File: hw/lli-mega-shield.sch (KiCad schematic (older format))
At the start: 39 parts

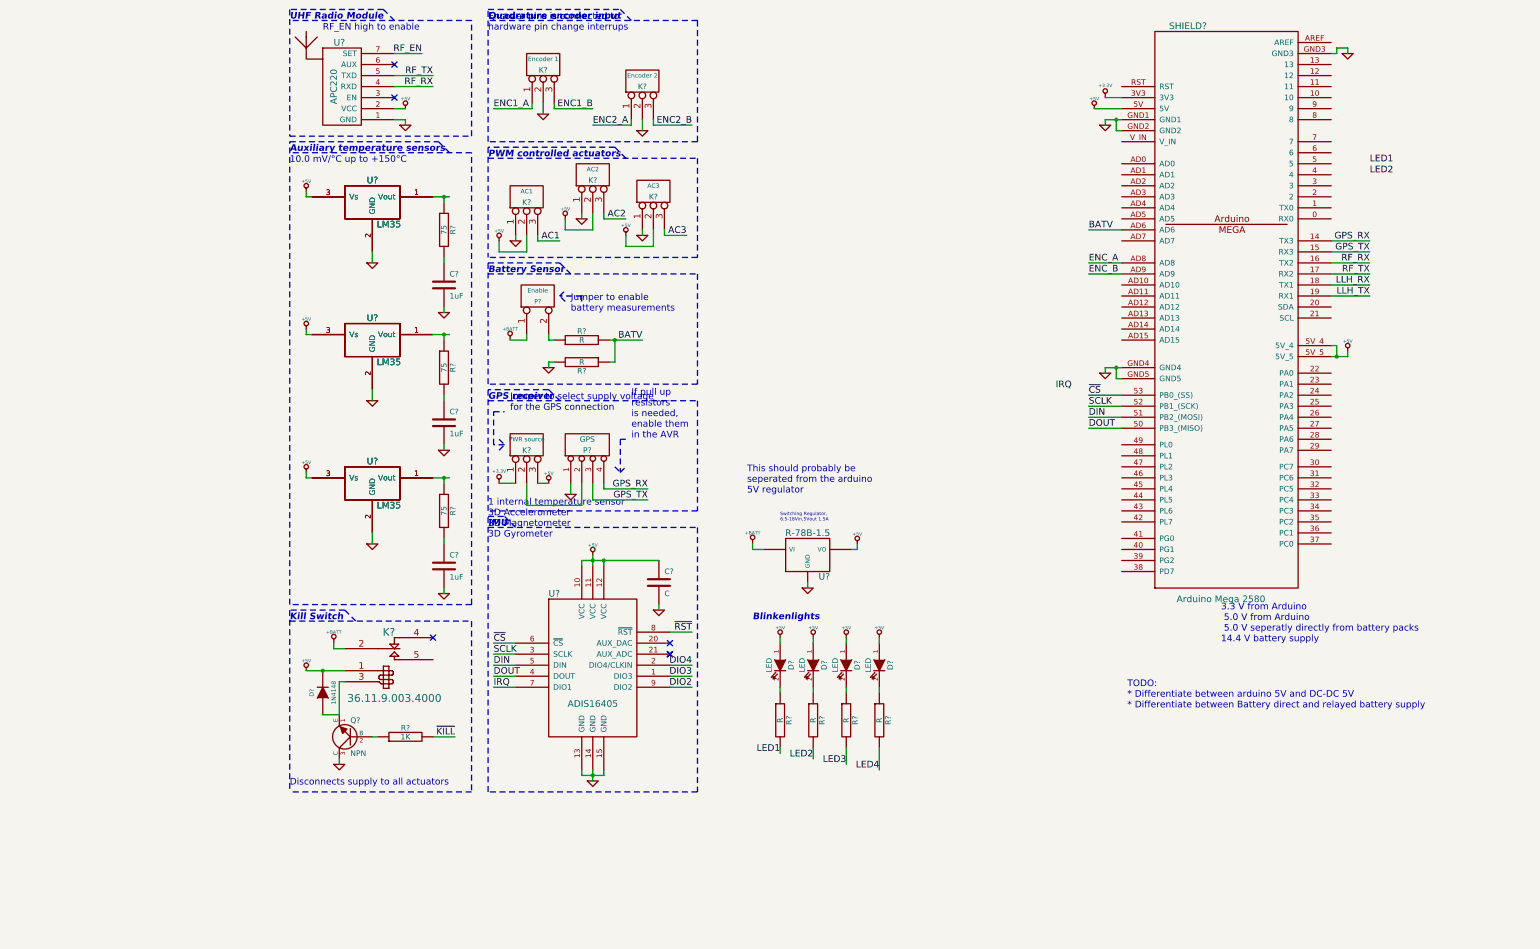
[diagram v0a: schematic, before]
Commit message: That must be hardware enough today
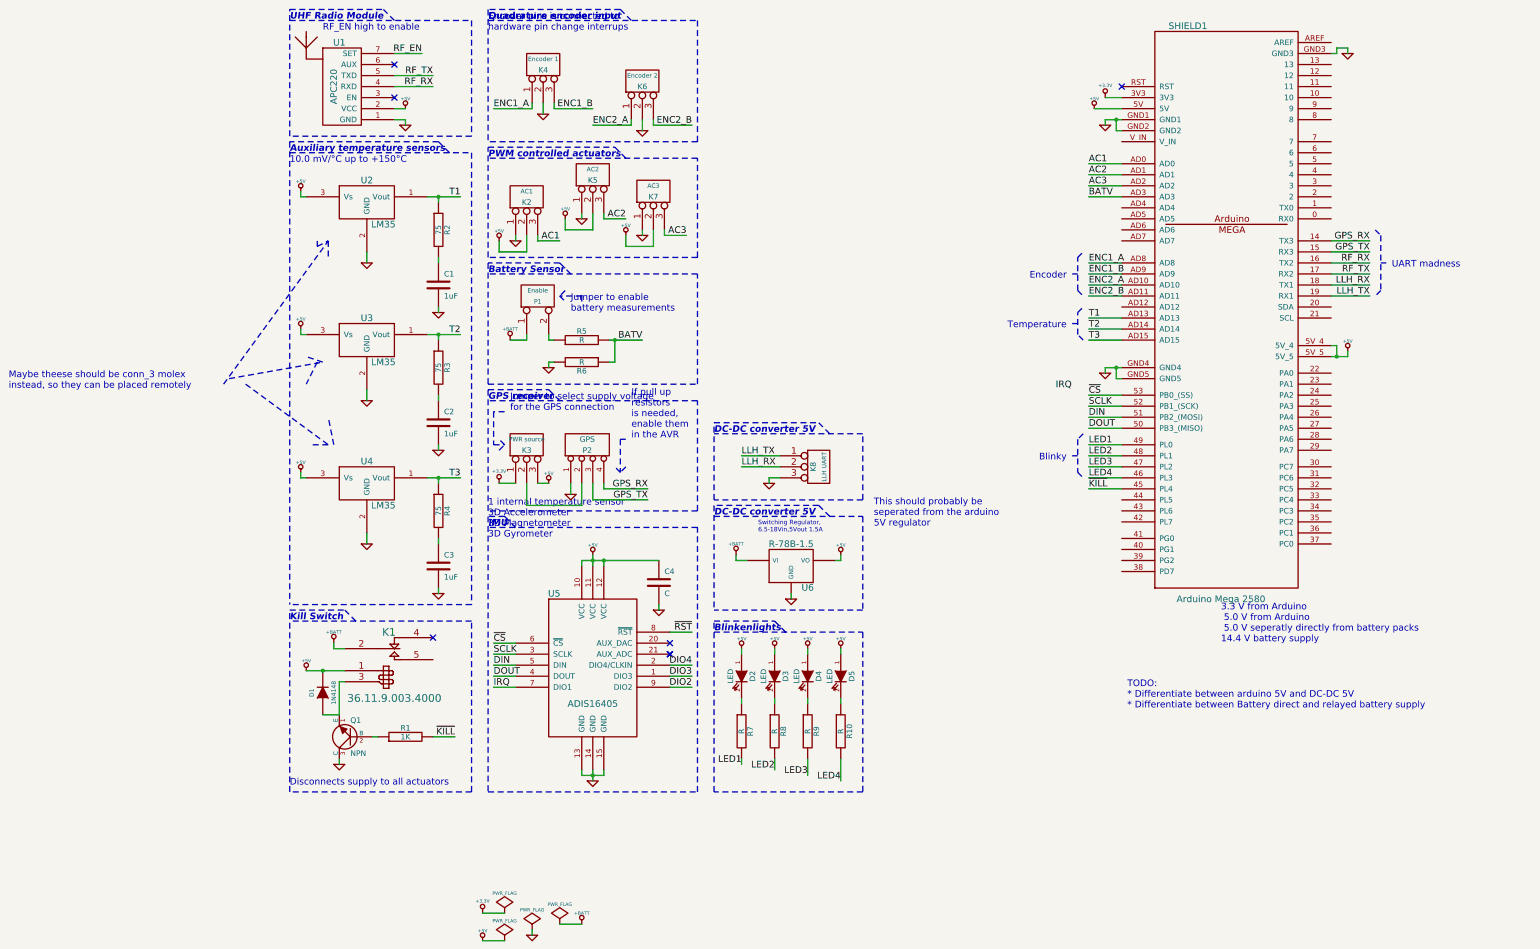
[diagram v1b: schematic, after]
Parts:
- removed U? (x3): LM35, symbol LM35
- added K8: LLH UART, symbol CONN_3
- gave numbers to parts that had none: 36
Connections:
- net ENC_A is gone; now on net ENC1_A: SHIELD1.AD8
- net ENC_B is gone; now on net ENC1_B: SHIELD1.AD9
- net AC1: now also SHIELD1.AD0
- net AC2: now also SHIELD1.AD1
- net AC3: now also SHIELD1.AD2
- net BATV: now also SHIELD1.AD3; no longer SHIELD1.AD6
- net ENC2_A: now also SHIELD1.AD10
- net ENC2_B: now also SHIELD1.AD11
- net GND: now also K8.3 (P3)
- net LED1: now also SHIELD1.49 (PL0)
- net LED2: now also SHIELD1.48 (PL1)
- net LED3: now also SHIELD1.47 (PL2)
- net LED4: now also SHIELD1.46 (PL3)
- net LLH_RX: now also K8.2 (PM)
- net LLH_TX: now also K8.1 (P1)
- net ~KILL: now also SHIELD1.45 (PL4)
- net T1: now reaches SHIELD1.AD13
- net T1: now also R2.1, U2.1 (Vout)
- net T2: now reaches SHIELD1.AD14
- net T2: now also R3.1, U3.1 (Vout)
- net T3: now reaches SHIELD1.AD15
- net T3: now also R4.1, U4.1 (Vout)
- no-connect marks 6 -> 7
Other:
- note added: "Blinky"
- note added: "DC-DC converter 5V"
- note added: "Encoder"
- note added: "Maybe theese should be conn_3 molex\ninstead, so they can be placed remotely"
- note added: "Temperature"
- note added: "UART madness"
- moved on the sheet: C1, C2, C3, D2, D3, D4, D5, R10, R2, R3, R4, R7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
